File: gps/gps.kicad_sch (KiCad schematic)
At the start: 19 parts, among them J1 I2C, J2 I2C, J3 USB_pads, U1 NEO-M9N, U2 TPS613226ADBVR

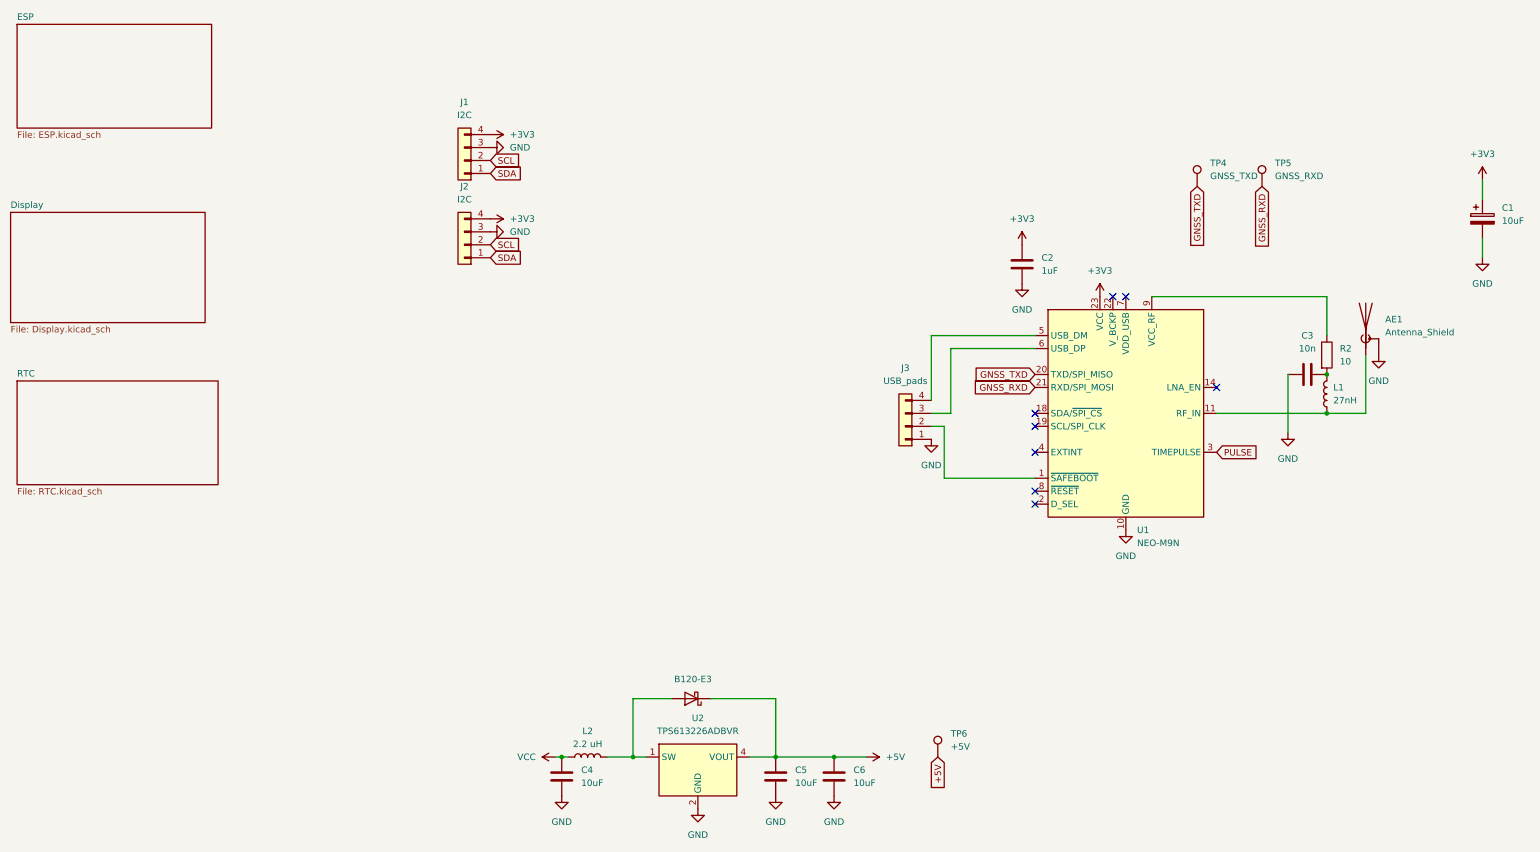
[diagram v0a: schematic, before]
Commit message: update
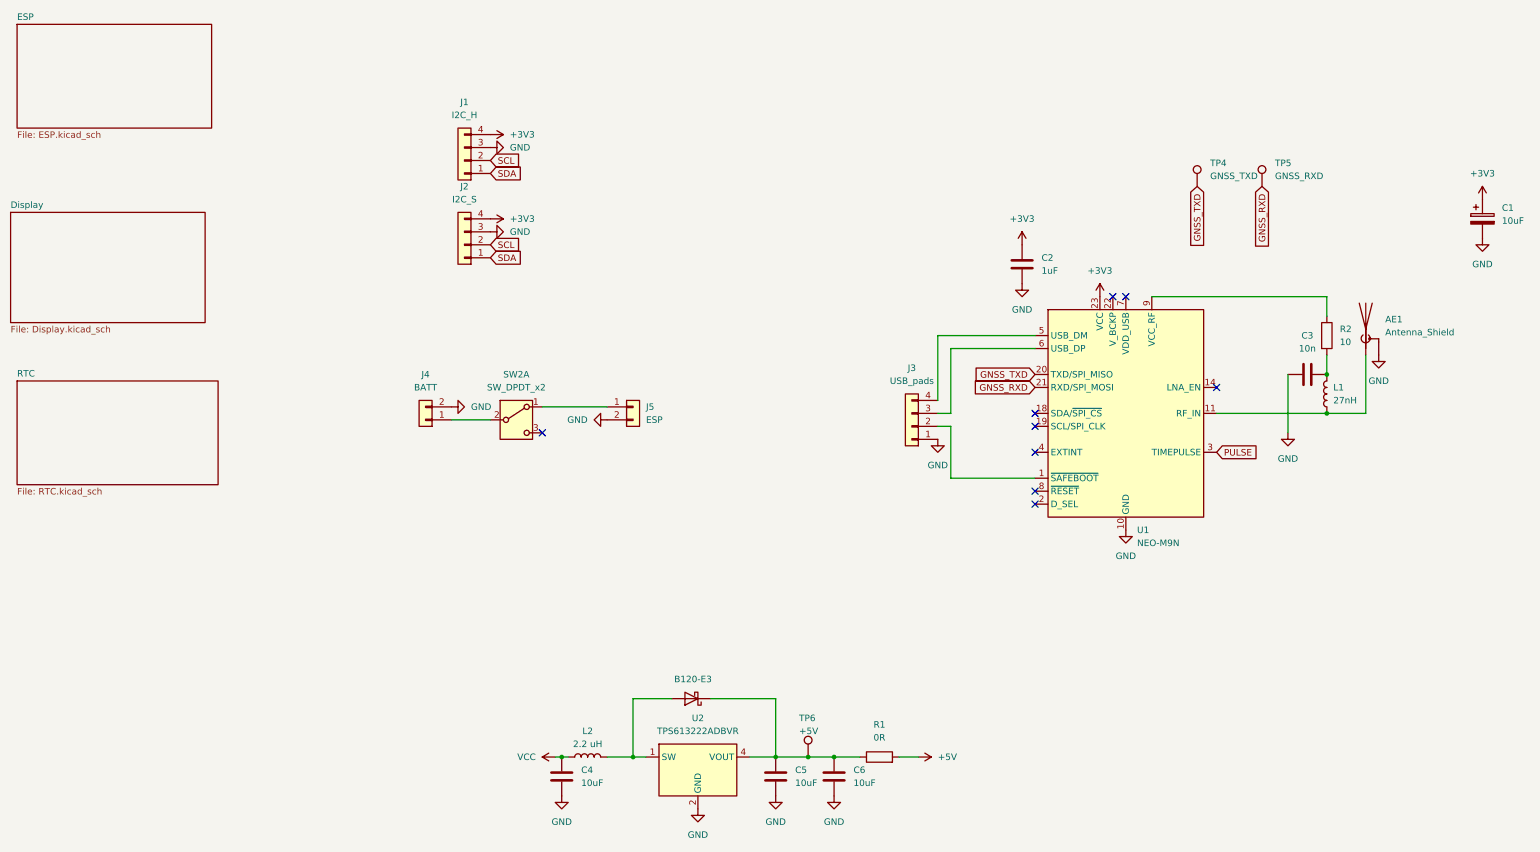
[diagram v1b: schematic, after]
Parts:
- added J4: BATT, 1769:1769, symbol Connector_Generic:Conn_01x02
- added J5: ESP, Connector_PinSocket_2.54mm:PinSocket_1x02_P2.54mm_Vertical, symbol Connector_Generic:Conn_01x02
- added R1: 0R, Resistor_SMD:R_0805_2012Metric_Pad1.20x1.40mm_HandSolder, symbol Device:R
- added SW2: SW_DPDT_x2, Button_Switch_THT:MSN22AFW01, symbol Switch:SW_DPDT_x2
- J1: value I2C -> I2C_H
- J2: value I2C -> I2C_S
- U2: value TPS613226ADBVR -> TPS613222ADBVR
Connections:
- net +5V: now also R1.2; no longer C5.1, C6.1, D2.1 (K), TP6.1, U2.4 (VOUT)
- net GND: now also J4.2 (Pin_2), J5.2 (Pin_2)
- new net: C5.1, C6.1, D2.1 (K), R1.1, TP6.1, U2.4 (VOUT)
- new net: J5.1 (Pin_1), SW2.1 (A)
- new net: J4.1 (Pin_1), SW2.2 (B)
- no-connect marks 8 -> 9
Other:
- moved on the sheet: J3, R2, TP6

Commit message: PCB-update
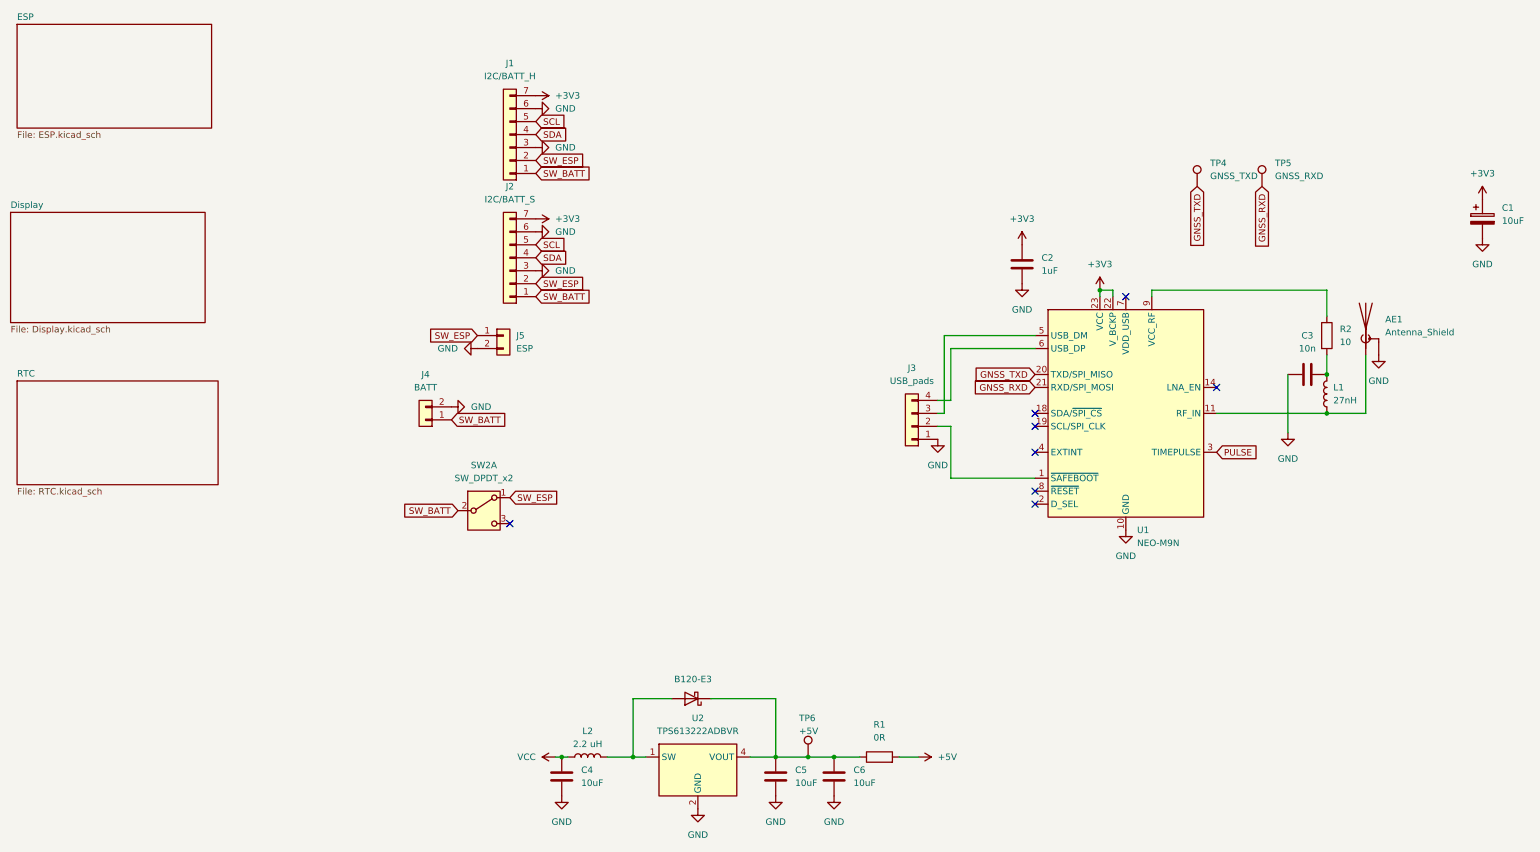
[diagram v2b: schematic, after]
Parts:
- removed J1: I2C_H, Connector_PinHeader_2.54mm:PinHeader_1x04_P2.54mm_Vertical, symbol Connector_Generic:Conn_01x04
- removed J2: I2C_S, Connector_PinSocket_2.54mm:PinSocket_1x04_P2.54mm_Vertical, symbol Connector_Generic:Conn_01x04
- added J1: I2C/BATT_H, Connector_PinHeader_2.54mm:PinHeader_1x07_P2.54mm_Vertical, symbol Connector_Generic:Conn_01x07
- added J2: I2C/BATT_S, Connector_PinSocket_2.54mm:PinSocket_1x07_P2.54mm_Vertical, symbol Connector_Generic:Conn_01x07
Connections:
- net +3V3: now also U1.22 (V_BCKP), J1.7 (Pin_7), J2.7 (Pin_7)
- net GND: now also J1.3 (Pin_3), J1.6 (Pin_6), J2.3 (Pin_3), J2.6 (Pin_6)
- net SCL: now also J1.5 (Pin_5), J2.5 (Pin_5)
- net SDA: now also J1.4 (Pin_4), J2.4 (Pin_4)
- net at J3.3 (Pin_3): now also U1.5 (USB_DM); no longer U1.6 (USB_DP)
- net at J3.4 (Pin_4): now also U1.6 (USB_DP); no longer U1.5 (USB_DM)
- net SW_ESP: now reaches J5.1 (Pin_1), SW2.1 (A)
- net SW_ESP: now also J1.2 (Pin_2), J2.2 (Pin_2)
- net SW_BATT: now reaches J4.1 (Pin_1), SW2.2 (B)
- net SW_BATT: now also J1.1 (Pin_1), J2.1 (Pin_1)
- no-connect marks 9 -> 8
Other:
- moved on the sheet: J5, SW2A
